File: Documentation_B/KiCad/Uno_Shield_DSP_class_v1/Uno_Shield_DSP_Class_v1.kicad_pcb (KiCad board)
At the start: 2 copper layers, 68.6 x 53.3 mm, 46 parts, among them J1 Power, J10 AudioJack5, J11 AudioJack5, J12 AUDIO_IN, J2 Digital/PWM, J3 Analog, J4 Digital/PWM, J5 IMU_CONN, J6 SCREEN_CONN, J7 AUDIO_OUT, J9 JUMPER, SW1 BT_1, SW2 BT_2, U1 MCP6002-xP

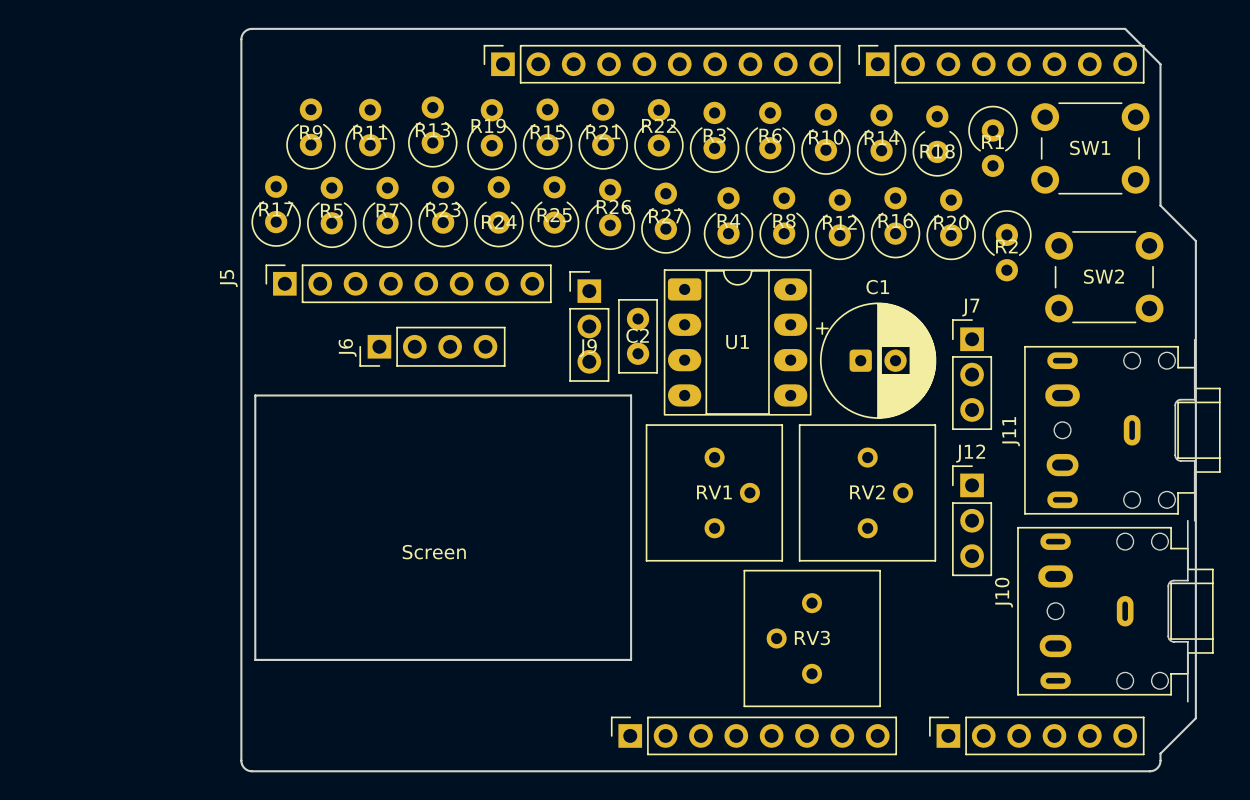
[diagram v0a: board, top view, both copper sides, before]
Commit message: Add files via upload
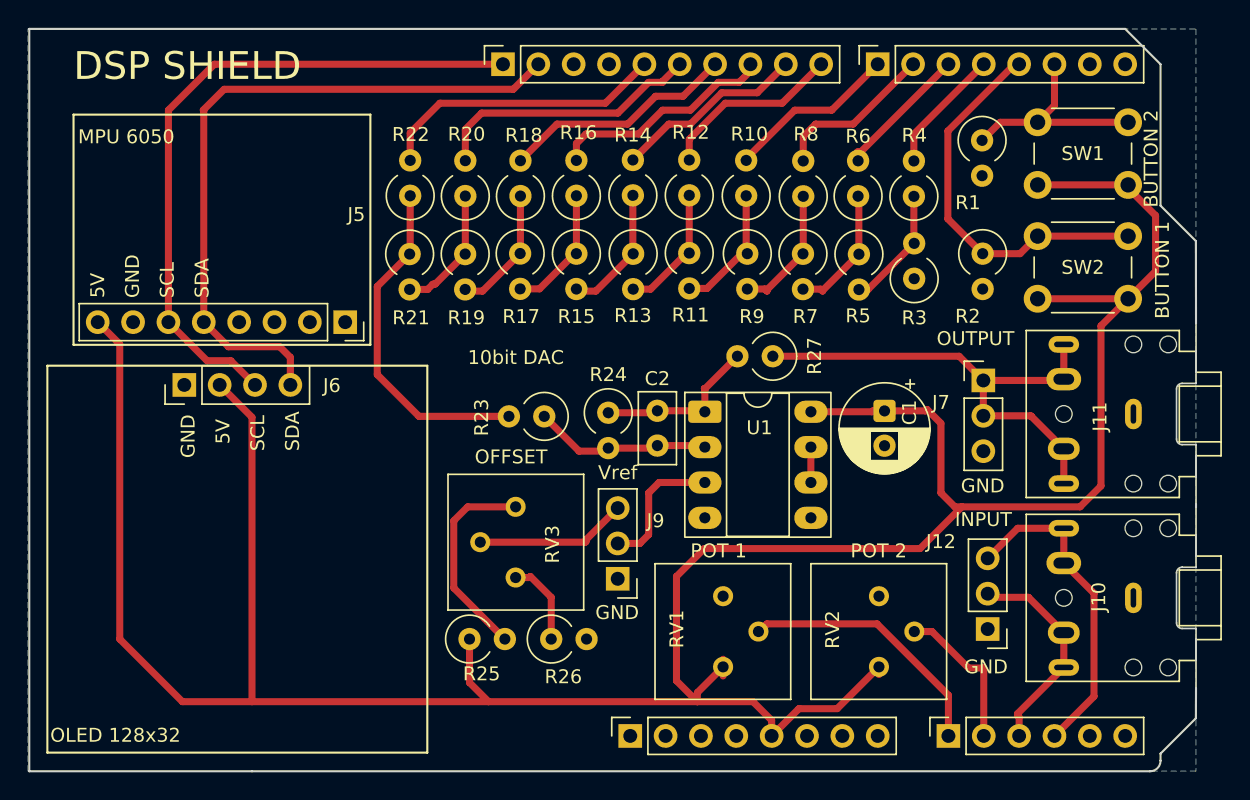
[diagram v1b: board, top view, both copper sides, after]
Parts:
- added G***: LOGO, LOGO, B.Cu at (98.3, 56.1)
- C1: footprint Capacitor_THT:CP_Radial_D8.0mm_P2.50mm -> Capacitor_THT:CP_Radial_D6.3mm_P2.50mm
- moved R5 37.9 mm to (144.4, 62.9), turned to -90 degrees
- moved R20 35.0 mm to (116.1, 58.7)
- moved R9 32.3 mm to (136.3, 62.8), turned to -90 degrees
- moved R25 30.5 mm to (116.4, 90.5), turned to 0 degrees
- moved R18 30.1 mm to (120.0, 58.7)
- moved R26 30.0 mm to (122.3, 90.5), turned to 0 degrees
- moved R7 29.9 mm to (140.3, 62.8), turned to -90 degrees
- moved R11 24.2 mm to (132.2, 62.8), turned to -90 degrees
- moved R16 23.1 mm to (124.1, 58.6)
- moved RV3 22.4 mm to (119.7, 81.0)
- moved J9 20.8 mm to (127.0, 86.2), turned to 180 degrees
- moved R22 18.2 mm to (112.1, 58.6)
- moved R14 18.2 mm to (128.1, 58.6)
- moved R17 17.7 mm to (120.0, 62.8), turned to -90 degrees
- moved R3 17.1 mm to (148.3, 64.6)
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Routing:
- net +5V: track 0.00 -> 214.0 mm
- net /SDA: track 0.00 -> 49.9 mm
- net /SCL: track 0.00 -> 48.7 mm
- net /AUDIO_OUT: track 0.00 -> 36.0 mm
- net /BT2: track 0.00 -> 28.1 mm
- net Net-(R21-Pad1): track 0.00 -> 24.5 mm
- net /IN_LEFT: track 0.00 -> 23.4 mm
- net /D9: track 0.00 -> 20.8 mm
- net /D8: track 0.00 -> 19.6 mm
- net /A0: track 0.00 -> 18.9 mm
- net /D7: track 0.00 -> 16.9 mm
- net /D6: track 0.00 -> 16.4 mm
- net /BT1: track 0.00 -> 15.7 mm
- net /IN_RIGHT: track 0.00 -> 15.5 mm
- net Net-(R25-Pad2): track 0.00 -> 14.9 mm
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- added copper zone on B.Cu, net GND
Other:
- board size 68.6 x 53.3 mm -> 83.8 x 53.3 mm
- board text added: "10bit DAC"
- board text added: "5V"
- board text added: "BUTTON 1"
- board text added: "BUTTON 2"
- board text added: "DSP SHIELD"
- board text added: "GND"
- board text added: "INPUT"
- board text added: "MPU 6050"
- board text added: "OFFSET"
- board text added: "OLED 128x32"
- board text added: "OUTPUT"
- board text added: "POT 1"
- board text added: "POT 2"
- board text added: "SCL"
- board text added: "SDA"
- board text added: "Spencer Lu February 2026 Version 1"
- board text added: "Vref"
- board text removed: "ICSP"
- board text removed: "Screen"
